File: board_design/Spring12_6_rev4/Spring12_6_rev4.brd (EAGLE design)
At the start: 100 x 80.6 mm, 48 parts, among them IC1 LM555D, J3 PICKIT, Q1 20MHz, SW0 SW-PB-MOM

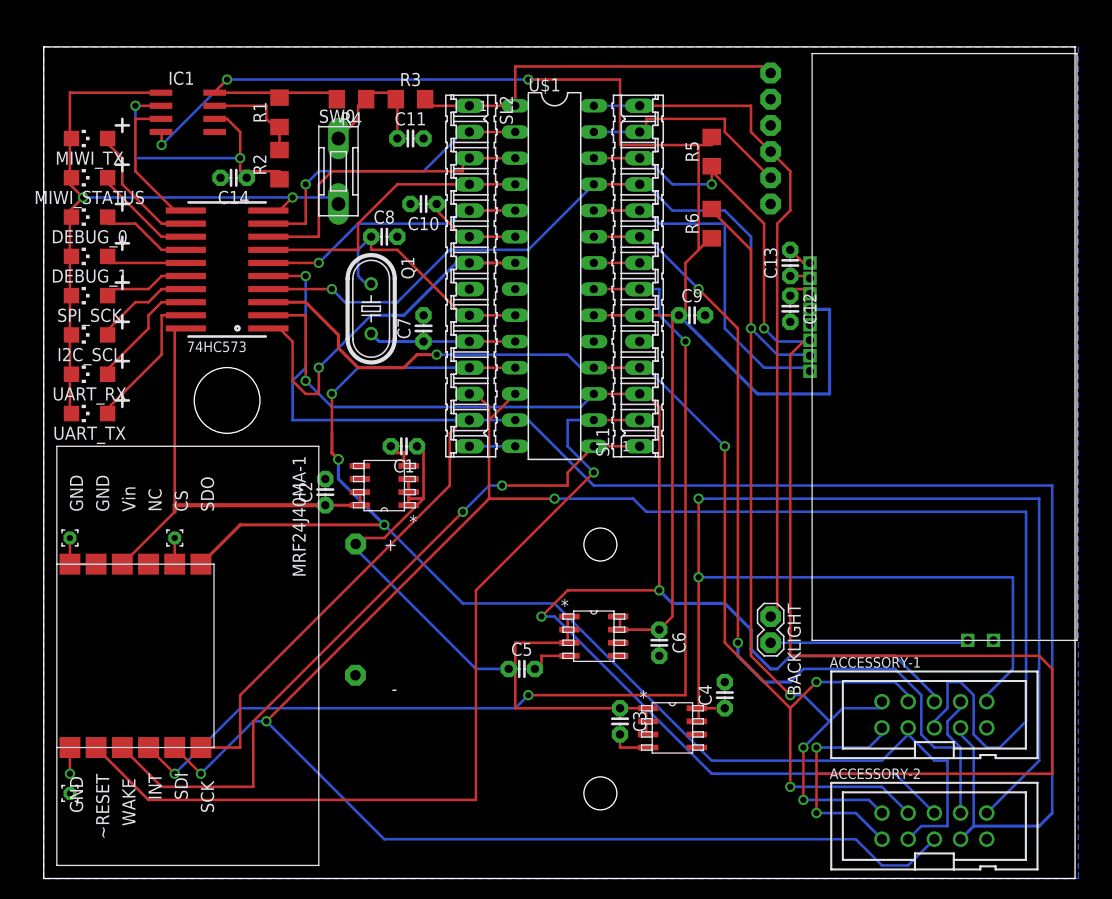
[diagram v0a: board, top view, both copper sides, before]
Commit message: board design... hopefully done
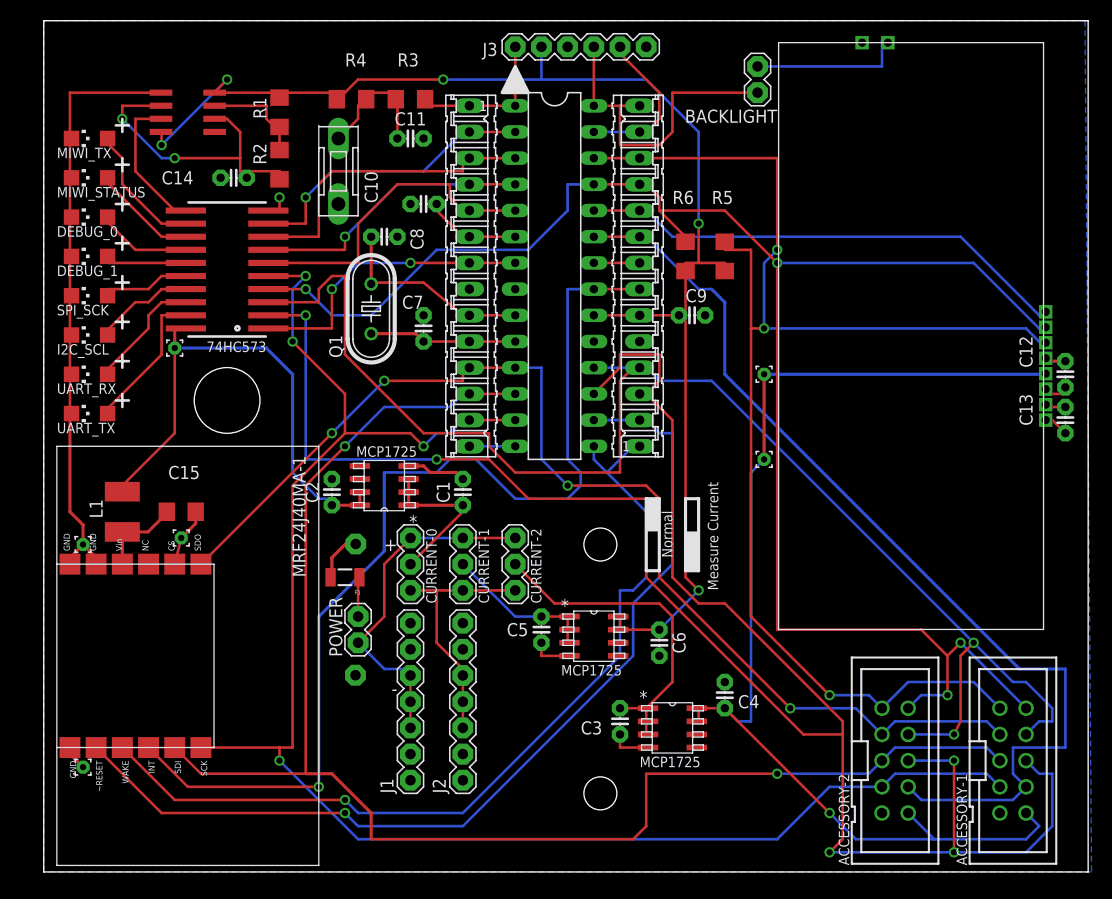
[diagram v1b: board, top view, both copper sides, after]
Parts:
- added C15: 100pF, rcl:C1206
- added F1: 1A PTC, SparkFun:PTC-1206
- added J1, J2: (no value), 4534:MA07-1
- added L1: 10nH, rcl:L1812
- added POWER: MA02-1, 4534:MA02-1
- added SV3, SV4, SV5: (no value), 4534:MA03-1
- added U$3, U$4, U$5: VIA, 4534_I2C2:VIA
- R5, R6: value 4K7 -> 10K
- U$2: value NHD-C0216CIZ-FN-FBW-3V -> NHD-C0216CIZ-FSW-FBW-3V3
- moved BACKLIGHT 53.4 mm to (69.2, 77.5), turned to 90 degrees
- moved C13 30.7 mm to (99.1, 44.5), turned to 270 degrees
- moved U$2 27.5 mm to (97.2, 44.5), turned to 90 degrees
- moved C12 27.4 mm to (99.1, 48.9), turned to 90 degrees
- moved J3 20.4 mm to (52.1, 80.6), flipped to the top, turned to 0 degrees
- moved R5 10.2 mm to (66.0, 60.3), turned to 270 degrees
- moved ACCESSORY-1 8.82 mm to (94.0, 11.4), turned to 270 degrees
- moved ACCESSORY-2 7.41 mm to (82.5, 11.4), turned to 270 degrees
- moved C1 7.24 mm to (40.6, 37.5), turned to 90 degrees
- moved C5 4.26 mm to (48.3, 24.1), turned to 270 degrees
- moved R6 4.07 mm to (62.2, 60.3)
- moved U$18 2.84 mm to (3.81, 10.8)
- moved U$19 1.42 mm to (3.81, 32.4)
- moved C2 0.64 mm to (27.9, 37.5)
- moved U$20 0.64 mm to (13.3, 33.0)
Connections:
- removed net 5V: J3.2
- new net BATT: BATT0.P$2, F1.2
- new net CURRENT: J2.3, J2.4, J2.5, SV3.1, SV4.1, SV5.1
- new net MIWI-VDD: C15.1, L1.1, RF0.10
- new net N$12: F1.1, POWER.1
- new net N$14: J1.2
- new net N$17: J2.6
- new net N$21: J2.2
- new net N$7: J1.6
- new net VCC_REG0: C5.1, REG0.1, REG0.2, REG0.3, SV3.2
- new net VCC_REG1: C1.1, REG1.1, REG1.2, REG1.3, SV4.2
- new net VCC_REG2: C3.1, REG2.1, REG2.2, REG2.3, SV5.2
- net VCC_BATT: now also J1.3, J1.4, J1.5, POWER.2, SV3.3, SV4.3, SV5.3; no longer BATT0.P$2, C1.1, C3.1, C5.1, REG0.1, REG0.2, REG0.3, REG1.1, REG1.2, REG1.3, REG2.1, REG2.2, REG2.3
- net VDD_ACC: now also U$2.5, U$3.1, U$4.1
- net VDD_MIWI: now also L1.2, U$5.1; no longer RF0.10
- net VDD_PIC: now also J3.2; no longer U$2.5
- net VSS: now also C15.2, J1.1, J1.7, J2.1, J2.7
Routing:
- net SPI_MOSI: track 220.5 -> 144.3 mm, vias 3 -> 2
- net UART_TX: track 156.3 -> 197.3 mm, vias 3 -> 5
- net VDD_PIC: track 171.1 -> 135.2 mm, vias 3 -> 5
- net PGD: track 67.5 -> 31.6 mm
- net VCC_BATT: track 69.9 -> 34.3 mm
- net VCC_REG2: track 0.00 -> 32.9 mm
- net SPI_SCK: track 191.3 -> 158.5 mm, vias 1 -> 4
- net CURRENT: track 0.00 -> 24.5 mm
- net VDD_ACC: track 133.7 -> 110.4 mm, vias 2 -> 1
- net UART_RX: track 113.6 -> 136.8 mm, vias 4 -> 2
- net MCLR: track 38.4 -> 15.3 mm
- net SPI_MISO: track 130.5 -> 111.6 mm, vias 3 -> 4
- net I2C_SCL: track 148.1 -> 165.8 mm, vias 5 -> 4
- net MRF-WAKE: track 69.9 -> 85.7 mm, vias 2 -> 1
- net I2C_SDA: track 148.4 -> 132.7 mm, vias 4 -> 3
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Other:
- board size 100 x 80.6 mm -> 101.3 x 82.5 mm
- board text added: "CURRENT-0"
- board text added: "CURRENT-1"
- board text added: "CURRENT-2"
- board text added: "MCP1725"
- board text added: "Measure Current"
- board text added: "Normal"
